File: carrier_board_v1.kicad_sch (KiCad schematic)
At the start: 0 parts

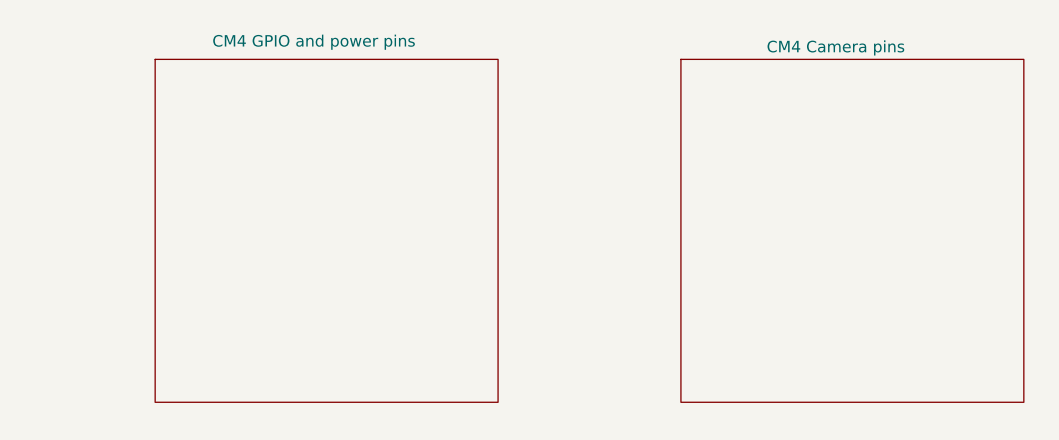
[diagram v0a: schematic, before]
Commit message: schematic complete
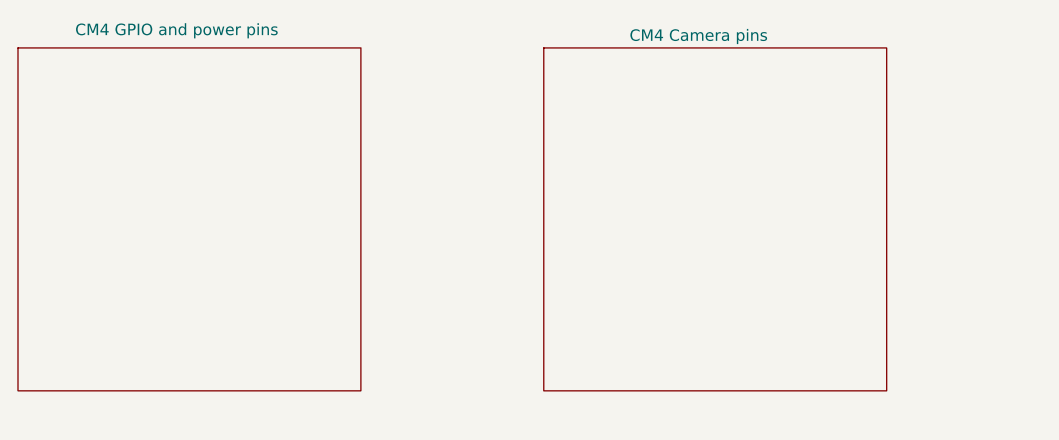
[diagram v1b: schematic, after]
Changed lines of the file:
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@@
     (comment 4 "Author: Iiro Karppanen")
   )
-  (sheet (at 113.665 45.085) (size 38.1 38.1)
+  (sheet (at 98.425 43.815) (size 38.1 38.1)
     (stroke (width 0) (type solid) (color 132 0 132 1))
     (fill (color 255 255 255 0.0000))
-    (property "Sheetname" "CM4 Camera pins" (at 123.19 44.45 0)
+    (property "Sheetname" "CM4 Camera pins" (at 107.95 43.18 0)
       (effects (font (size 1.27 1.27)) (justify left bottom))
     )
-    (property "Sheetfile" "cm4-high-speed.kicad_sch" (at 113.665 83.6935 0)
+    (property "Sheetfile" "cm4-high-speed.kicad_sch" (at 98.425 82.4235 0)
       (effects (font (size 1.27 1.27)) (justify left top) hide)
     )
@@
     )
   )
-  (sheet (at 55.245 45.085) (size 38.1 38.1)
+  (sheet (at 40.005 43.815) (size 38.1 38.1)
     (stroke (width 0) (type solid) (color 132 0 132 1))
     (fill (color 255 255 255 0.0000))
-    (property "Sheetname" "CM4 GPIO and power pins" (at 61.595 43.815 0)
+    (property "Sheetname" "CM4 GPIO and power pins" (at 46.355 42.545 0)
       (effects (font (size 1.27 1.27)) (justify left bottom))
     )
-    (property "Sheetfile" "cm4-gpio.kicad_sch" (at 55.245 83.6935 0)
+    (property "Sheetfile" "cm4-gpio.kicad_sch" (at 40.005 82.4235 0)
       (effects (font (size 1.27 1.27)) (justify left top) hide)
     )

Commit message: pää hajoo
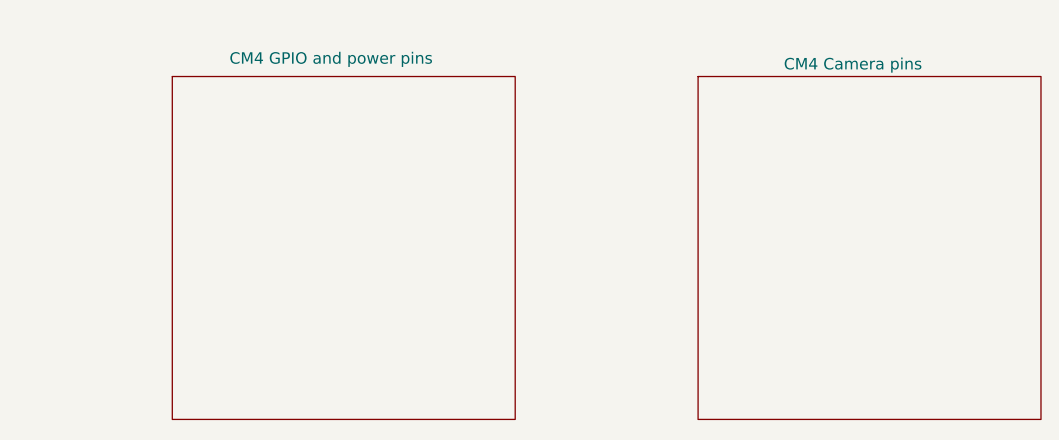
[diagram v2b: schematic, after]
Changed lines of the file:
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@@
     (comment 4 "Author: Iiro Karppanen")
   )
-  (sheet (at 98.425 43.815) (size 38.1 38.1)
+  (sheet (at 115.57 46.99) (size 38.1 38.1)
     (stroke (width 0) (type solid) (color 132 0 132 1))
     (fill (color 255 255 255 0.0000))
-    (property "Sheetname" "CM4 Camera pins" (at 107.95 43.18 0)
+    (property "Sheetname" "CM4 Camera pins" (at 125.095 46.355 0)
       (effects (font (size 1.27 1.27)) (justify left bottom))
     )
-    (property "Sheetfile" "cm4-high-speed.kicad_sch" (at 98.425 82.4235 0)
+    (property "Sheetfile" "cm4-high-speed.kicad_sch" (at 115.57 85.5985 0)
       (effects (font (size 1.27 1.27)) (justify left top) hide)
     )
@@
     )
   )
-  (sheet (at 40.005 43.815) (size 38.1 38.1)
+  (sheet (at 57.15 46.99) (size 38.1 38.1)
     (stroke (width 0) (type solid) (color 132 0 132 1))
     (fill (color 255 255 255 0.0000))
-    (property "Sheetname" "CM4 GPIO and power pins" (at 46.355 42.545 0)
+    (property "Sheetname" "CM4 GPIO and power pins" (at 63.5 45.72 0)
       (effects (font (size 1.27 1.27)) (justify left bottom))
     )
-    (property "Sheetfile" "cm4-gpio.kicad_sch" (at 40.005 82.4235 0)
+    (property "Sheetfile" "cm4-gpio.kicad_sch" (at 57.15 85.5985 0)
       (effects (font (size 1.27 1.27)) (justify left top) hide)
     )

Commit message: version3 complete
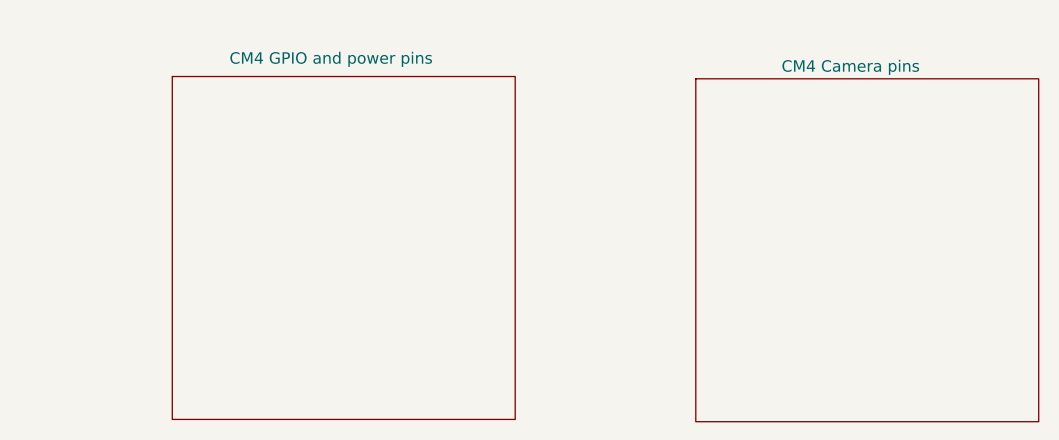
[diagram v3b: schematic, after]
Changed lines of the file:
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@@
     (comment 4 "Author: Iiro Karppanen")
   )
-  (sheet (at 115.57 46.99) (size 38.1 38.1)
+  (sheet (at 115.316 47.244) (size 38.1 38.1)
     (stroke (width 0) (type solid) (color 132 0 132 1))
     (fill (color 255 255 255 0.0000))
-    (property "Sheetname" "CM4 Camera pins" (at 125.095 46.355 0)
+    (property "Sheetname" "CM4 Camera pins" (at 124.841 46.609 0)
       (effects (font (size 1.27 1.27)) (justify left bottom))
     )
-    (property "Sheetfile" "cm4-high-speed.kicad_sch" (at 115.57 85.5985 0)
+    (property "Sheetfile" "cm4-high-speed.kicad_sch" (at 115.316 85.8525 0)
       (effects (font (size 1.27 1.27)) (justify left top) hide)
     )
